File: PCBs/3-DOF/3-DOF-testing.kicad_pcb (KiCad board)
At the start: 4 copper layers, 97.1 x 53.8 mm, 83 parts, among them J1 Conn_02x07_Odd_Even, J11 HBB, J12 RS485, J13 HBB, J14 HBA, J15 HBA, J17 Servo1, J2 Conn_02x08_Odd_Even, J3 Conn_02x08_Odd_Even, J5 24Vin, J9 Laser Diode, Q1 QServoA, Q5 S8550, Q6 LaserDiodeT, U1 MAX485E, U2 LM7805_TO220, U3 LM7805_TO220

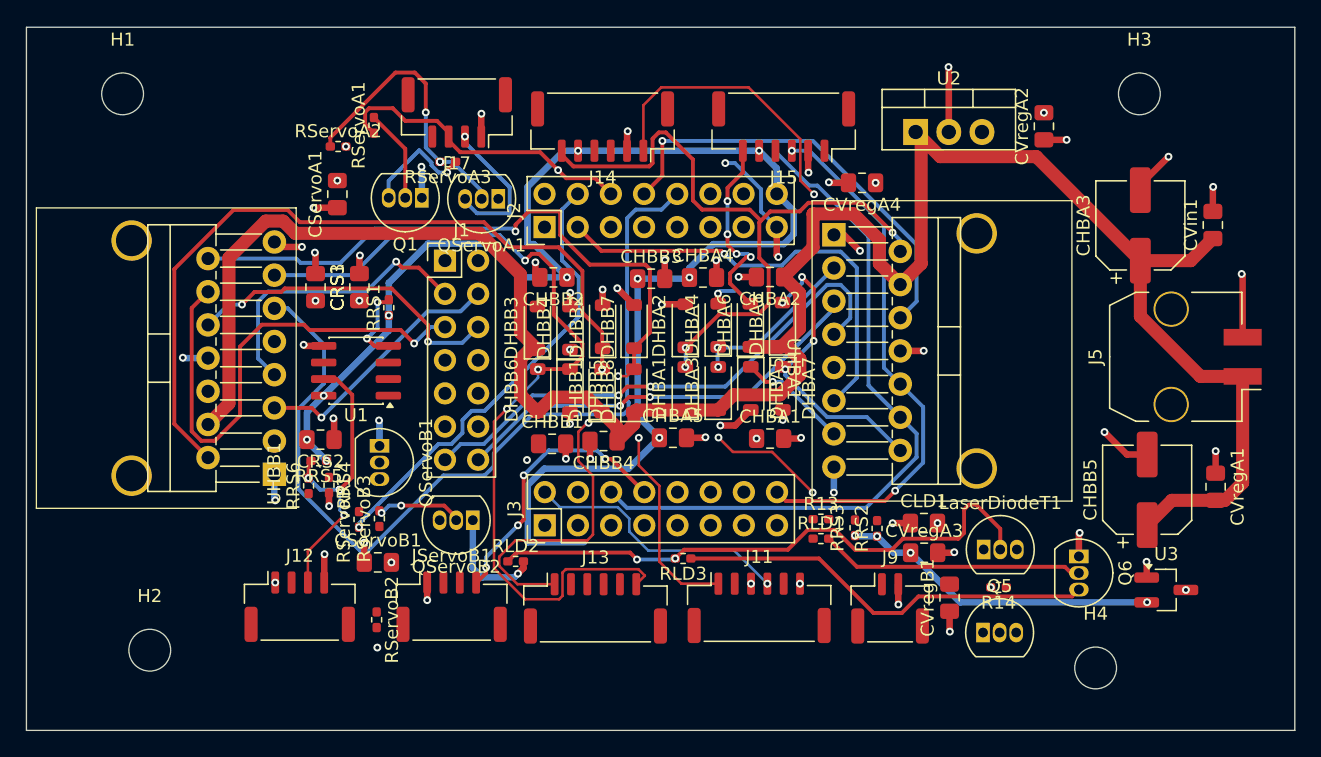
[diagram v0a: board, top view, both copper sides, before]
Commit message: see 3DOF-testing, routing rough draft
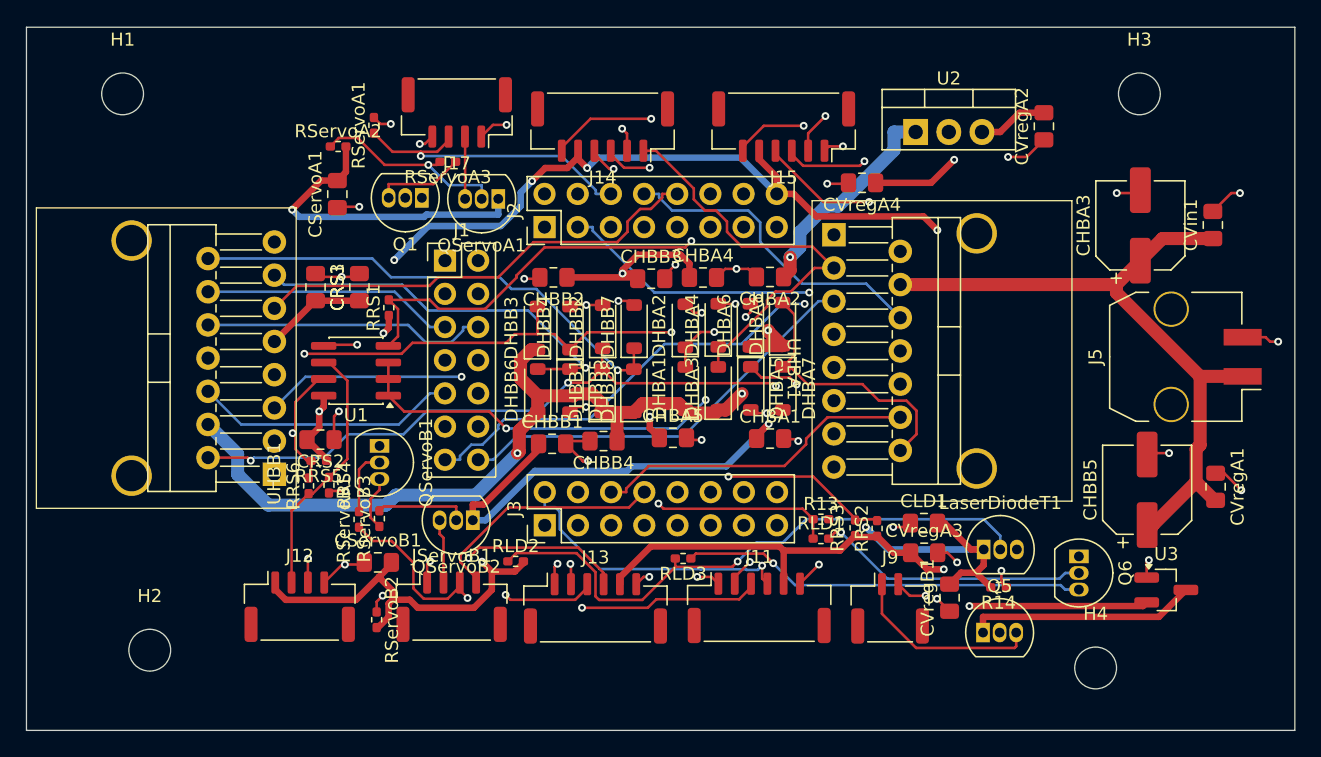
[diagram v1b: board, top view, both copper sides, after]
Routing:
- net /52: track 0.00 -> 64.6 mm, vias 0 -> 3
- net +3.3V: track 139.0 -> 189.3 mm, vias 14 -> 10
- net /26: track 0.00 -> 38.2 mm, vias 0 -> 1
- net /56: track 0.00 -> 35.5 mm, vias 0 -> 1
- net Net-(DHBB3-A): track 25.8 -> 60.9 mm, vias 2 -> 3
- net /55: track 68.4 -> 35.1 mm
- net /30: track 0.00 -> 33.2 mm, vias 0 -> 1
- net /51: track 5.92 -> 38.7 mm, vias 2 -> 1
- net /29: track 0.00 -> 30.8 mm, vias 0 -> 1
- net Net-(DHBB1-A): track 96.1 -> 65.7 mm
- net Net-(DHBA7-K): track 22.6 -> 47.5 mm, vias 4 -> 1
- net GND: track 101.9 -> 77.6 mm, vias 52 -> 36
- net /23: track 0.00 -> 24.3 mm, vias 0 -> 1
- net +5V: track 226.8 -> 248.3 mm, vias 15 -> 5
- net Net-(J9-Pin_1): track 0.00 -> 21.1 mm
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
